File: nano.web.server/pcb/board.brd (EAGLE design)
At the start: 88.7 x 59.4 mm, 9 parts, among them M1 ARDUINO-NANO-3.0

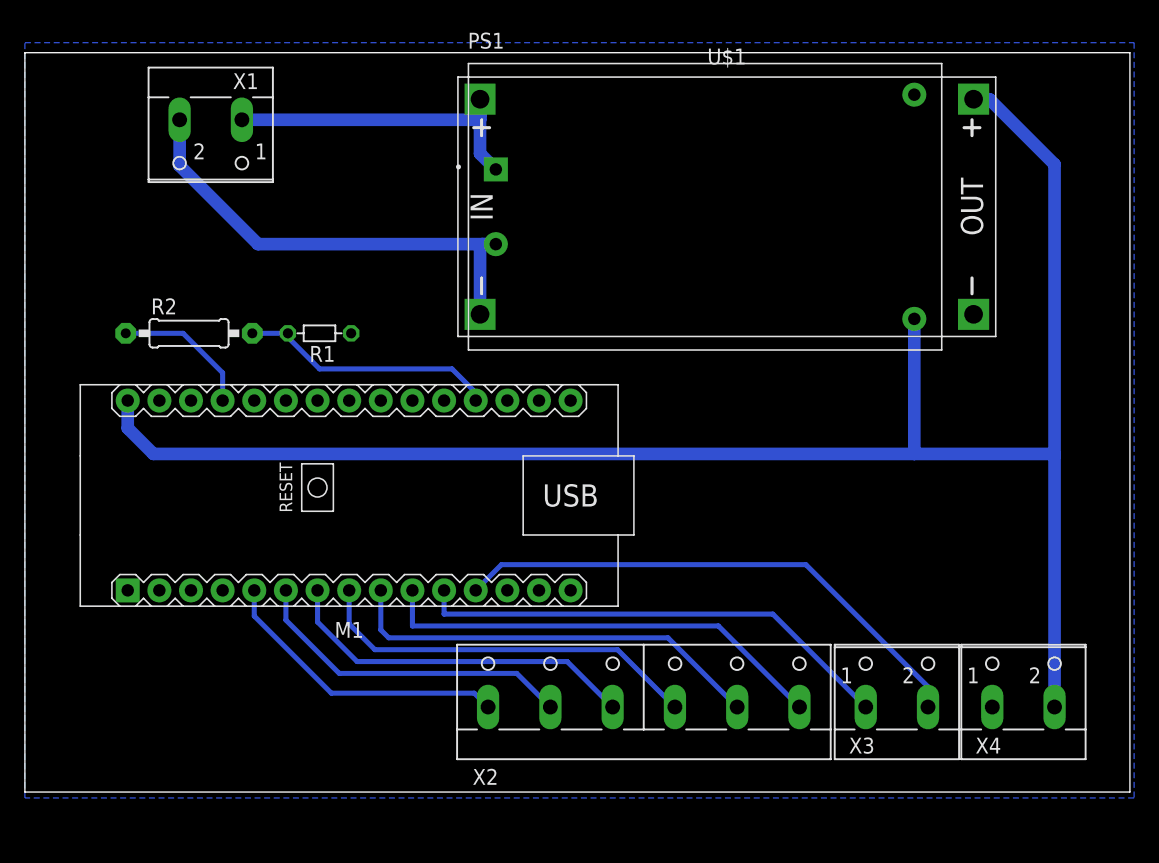
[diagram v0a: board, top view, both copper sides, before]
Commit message: board
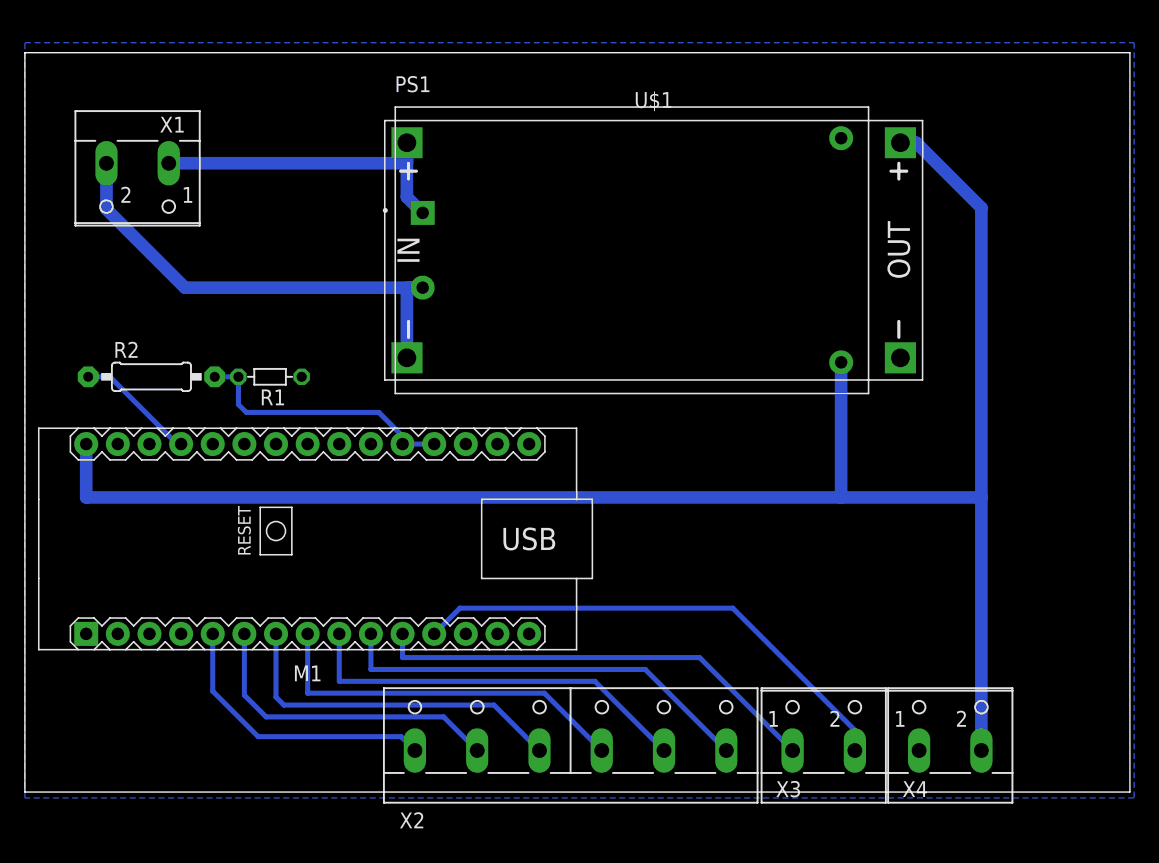
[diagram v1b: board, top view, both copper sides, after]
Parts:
- moved PS1 6.83 mm to (48.7, 43.5)
- moved U$1 6.83 mm to (50.5, 43.5)
- moved X2 6.83 mm to (43.8, 4.60)
- moved X3 6.83 mm to (64.1, 4.60)
- moved X4 6.83 mm to (74.3, 4.60)
- moved X1 6.83 mm to (9.05, 49.2)
- moved R1 5.29 mm to (19.7, 33.3)
- moved M1 4.83 mm to (22.7, 20.3)
- moved R2 4.61 mm to (10.2, 33.3)
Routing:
- net D9: track 42.9 -> 40.3 mm
- net D8: track 38.8 -> 36.3 mm
- net D7: track 36.6 -> 34.1 mm
- net D6: track 34.4 -> 32.2 mm
- net 5V: track 11.3 -> 9.70 mm
- net D5: track 31.6 -> 30.3 mm
- net VCC: track 140.6 -> 139.2 mm
- net D3: track 26.5 -> 25.5 mm
- net D2: track 23.9 -> 22.8 mm
- net D4: track 29.1 -> 28.0 mm
